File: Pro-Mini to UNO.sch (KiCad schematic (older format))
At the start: 16 parts, among them J1 DC 5.5x2.1mm, J2 JST 2pin, J3 2pin, U1 ARDUINO_Pro-Mini, U2 ARDUINO_UNOr3

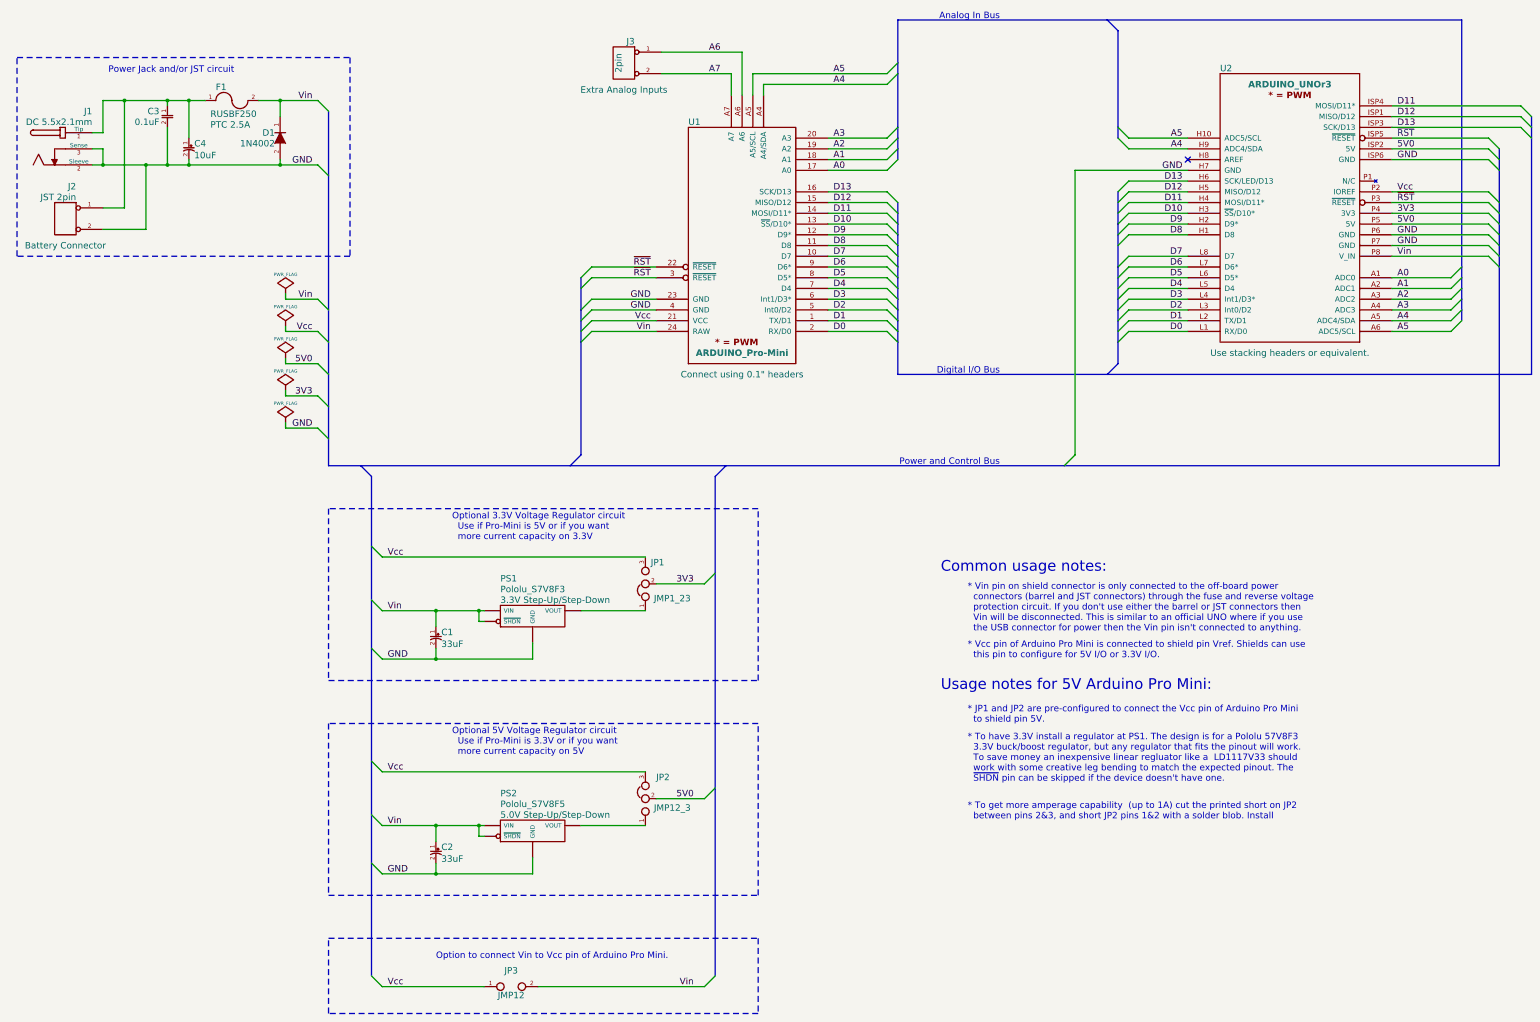
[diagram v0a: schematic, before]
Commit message: collected updates
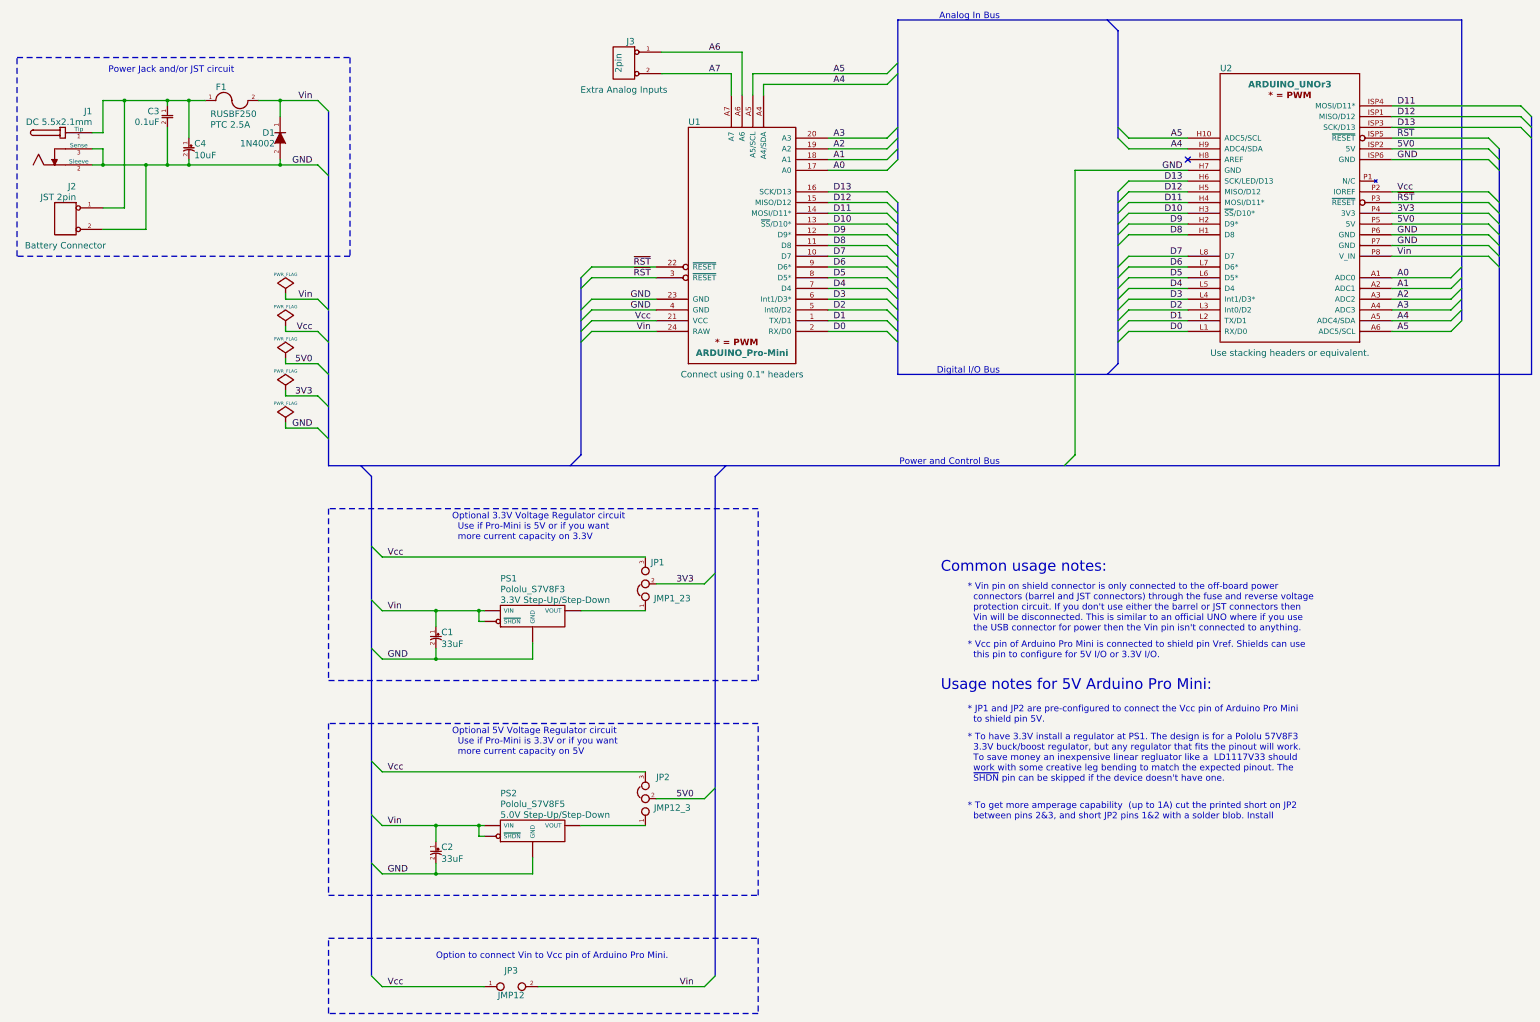
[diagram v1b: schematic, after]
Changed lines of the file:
@@
 	14000 1800 15200 1800
 Wire Bus Line
-	11450 2600 11450 2700
+	11450 2600 11450 4200
 Wire Bus Line
-	11450 2700 11450 2800
+	9400 2700 9400 4300
 Wire Bus Line
-	11450 2800 11450 2900
+	9400 1000 9400 2300
 Wire Bus Line
-	11450 2900 11450 3000
+	9400 1000 14650 1000
 Wire Bus Line
-	11450 3000 11450 3100
+	14650 1000 14650 3800
 Wire Bus Line
-	11450 3100 11450 3300
+	11450 1100 11450 2100
 Wire Bus Line
-	11450 3300 11450 3400
+	15300 4300 9400 4300
 Wire Bus Line
-	11450 3400 11450 3500
+	15300 1900 15300 4300
 Wire Bus Line
-	11450 3500 11450 3600
+	4100 5150 15000 5150
 Wire Bus Line
-	11450 3600 11450 3700
-Wire Bus Line
-	11450 3700 11450 3800
-Wire Bus Line
-	11450 3800 11450 3900
-Wire Bus Line
-	11450 3900 11450 4000
-Wire Bus Line
-	11450 4000 11450 4200
-Wire Bus Line
-	9400 2700 9400 2800
-Wire Bus Line
-	9400 2800 9400 2900
-Wire Bus Line
-	9400 2900 9400 3000
-Wire Bus Line
-	9400 3000 9400 3100
-Wire Bus Line
-	9400 3100 9400 3200
-Wire Bus Line
-	9400 3200 9400 3300
-Wire Bus Line
-	9400 3300 9400 3400
-Wire Bus Line
-	9400 3400 9400 3500
-Wire Bus Line
-	9400 3500 9400 3600
-Wire Bus Line
-	9400 3600 9400 3700
-Wire Bus Line
-	9400 3700 9400 3800
-Wire Bus Line
-	9400 3800 9400 3900
-Wire Bus Line
-	9400 3900 9400 4000
-Wire Bus Line
-	9400 4000 9400 4300
-Wire Bus Line
-	9400 1000 9400 1400
-Wire Bus Line
-	9400 1400 9400 1500
-Wire Bus Line
-	9400 1500 9400 2000
-Wire Bus Line
-	9400 2000 9400 2100
-Wire Bus Line
-	9400 2100 9400 2200
-Wire Bus Line
-	9400 2200 9400 2300
-Wire Bus Line
-	9400 1000 11350 1000
-Wire Bus Line
-	11350 1000 14650 1000
-Wire Bus Line
-	14650 1000 14650 3300
-Wire Bus Line
-	14650 3300 14650 3400
-Wire Bus Line
-	14650 3400 14650 3500
-Wire Bus Line
-	14650 3500 14650 3600
-Wire Bus Line
-	14650 3600 14650 3700
-Wire Bus Line
-	14650 3700 14650 3800
-Wire Bus Line
-	11450 1100 11450 2000
-Wire Bus Line
-	11450 2000 11450 2100
-Wire Bus Line
-	15300 4300 11350 4300
-Wire Bus Line
-	11350 4300 9400 4300
-Wire Bus Line
-	15300 1900 15300 2000
-Wire Bus Line
-	15300 2000 15300 2100
-Wire Bus Line
-	15300 2100 15300 4300
-Wire Bus Line
-	4100 5150 4400 5150
-Wire Bus Line
-	4400 5150 6350 5150
-Wire Bus Line
-	6350 5150 7800 5150
-Wire Bus Line
-	7800 5150 10950 5150
-Wire Bus Line
-	10950 5150 15000 5150
-Wire Bus Line
-	15000 2200 15000 2300
-Wire Bus Line
-	15000 2300 15000 2400
-Wire Bus Line
-	15000 2400 15000 2700
-Wire Bus Line
-	15000 2700 15000 2800
-Wire Bus Line
-	15000 2800 15000 2900
-Wire Bus Line
-	15000 2900 15000 3000
-Wire Bus Line
-	15000 3000 15000 3100
-Wire Bus Line
-	15000 3100 15000 3200
-Wire Bus Line
-	15000 3200 15000 3300
-Wire Bus Line
-	15000 3300 15000 5150
+	15000 2200 15000 5150
 Wire Wire Line
 	7200 1300 7950 1300
@@
 	7850 1500 7850 1700
 Wire Wire Line
-	1900 2350 2000 2350
-Wire Wire Line
-	2000 2350 2400 2350
-Wire Wire Line
-	2400 2350 2600 2350
-Wire Wire Line
-	2600 2350 2800 2350
-Wire Wire Line
-	2800 2350 3650 2350
-Wire Wire Line
-	3650 2350 4000 2350
+	1900 2350 4000 2350
 Wire Bus Line
-	4100 1850 4100 2450
+	4100 1850 4100 5150
 Wire Bus Line
-	4100 2450 4100 3700
-Wire Bus Line
-	4100 3700 4100 4000
-Wire Bus Line
-	4100 4000 4100 4300
-Wire Bus Line
-	4100 4300 4100 4600
-Wire Bus Line
-	4100 4600 4100 4900
-Wire Bus Line
-	4100 4900 4100 5150
-Wire Bus Line
-	6450 3400 6450 3500
-Wire Bus Line
-	6450 3500 6450 3700
-Wire Bus Line
-	6450 3700 6450 3800
-Wire Bus Line
-	6450 3800 6450 3900
-Wire Bus Line
-	6450 3900 6450 4000
-Wire Bus Line
-	6450 4000 6450 5050
+	6450 3400 6450 5050
 Wire Wire Line
 	3700 4450 3700 4500
@@
 	14000 2800 14900 2800
 Wire Bus Line
-	4500 5250 4500 5900
-Wire Bus Line
-	4500 5900 4500 6400
-Wire Bus Line
-	4500 6400 4500 6850
-Wire Bus Line
-	4500 6850 4500 7900
-Wire Bus Line
-	4500 7900 4500 8400
-Wire Bus Line
-	4500 8400 4500 8850
-Wire Bus Line
-	4500 8850 4500 9900
+	4500 5250 4500 9900
 Wire Wire Line
 	11050 2400 11050 5050
 Wire Wire Line
-	3450 1750 3650 1750
+	3450 1750 4000 1750
 Wire Wire Line
-	3650 1750 4000 1750
-Wire Wire Line
-	2000 1750 2200 1750
-Wire Wire Line
-	2200 1750 2600 1750
-Wire Wire Line
-	2600 1750 2800 1750
-Wire Wire Line
-	2800 1750 2950 1750
+	2000 1750 2950 1750
 Wire Wire Line
 	2000 1750 2000 2050
@@
 Connection ~ 2400 2350
 Wire Wire Line
-	4600 6950 5100 6950
-Wire Wire Line
-	5100 6950 6000 6950
+	4600 6950 6000 6950
 Wire Wire Line
 	6000 6950 6000 6800
@@
 	8100 7150 8100 5550
 Wire Wire Line
-	4600 8950 5100 8950
-Wire Wire Line
-	5100 8950 6000 8950
+	4600 8950 6000 8950
 Wire Wire Line
 	6000 8950 6000 8800
 Wire Wire Line
-	4600 8500 5100 8500
-Wire Wire Line
-	5100 8500 5500 8500
-Wire Wire Line
-	5500 8500 5550 8500
+	4600 8500 5550 8500
 Wire Wire Line
 	5550 8600 5500 8600
@@
 Connection ~ 5100 8950
 Wire Wire Line
-	4600 6500 5100 6500
-Wire Wire Line
-	5100 6500 5500 6500
-Wire Wire Line
-	5500 6500 5550 6500
+	4600 6500 5550 6500
 Wire Wire Line
 	7050 8000 4600 8000
@@
 	6550 3800 6450 3900
 Wire Bus Line
-	7700 5250 7700 6150
-Wire Bus Line
-	7700 6150 7700 8150
-Wire Bus Line
-	7700 8150 7700 9900
+	7700 5250 7700 9900
 Entry Bus Bus
 	7700 5250 7800 5150
